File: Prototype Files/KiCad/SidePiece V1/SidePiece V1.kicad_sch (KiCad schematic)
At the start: 32 parts, among them J1 USB_C_Receptacle_USB2.0_16P, J2 Conn_01x02, U1 RP2040, U2 NCP1117-3.3_SOT223, U3 W25Q128JVS, Y1 ABM8-272-T3

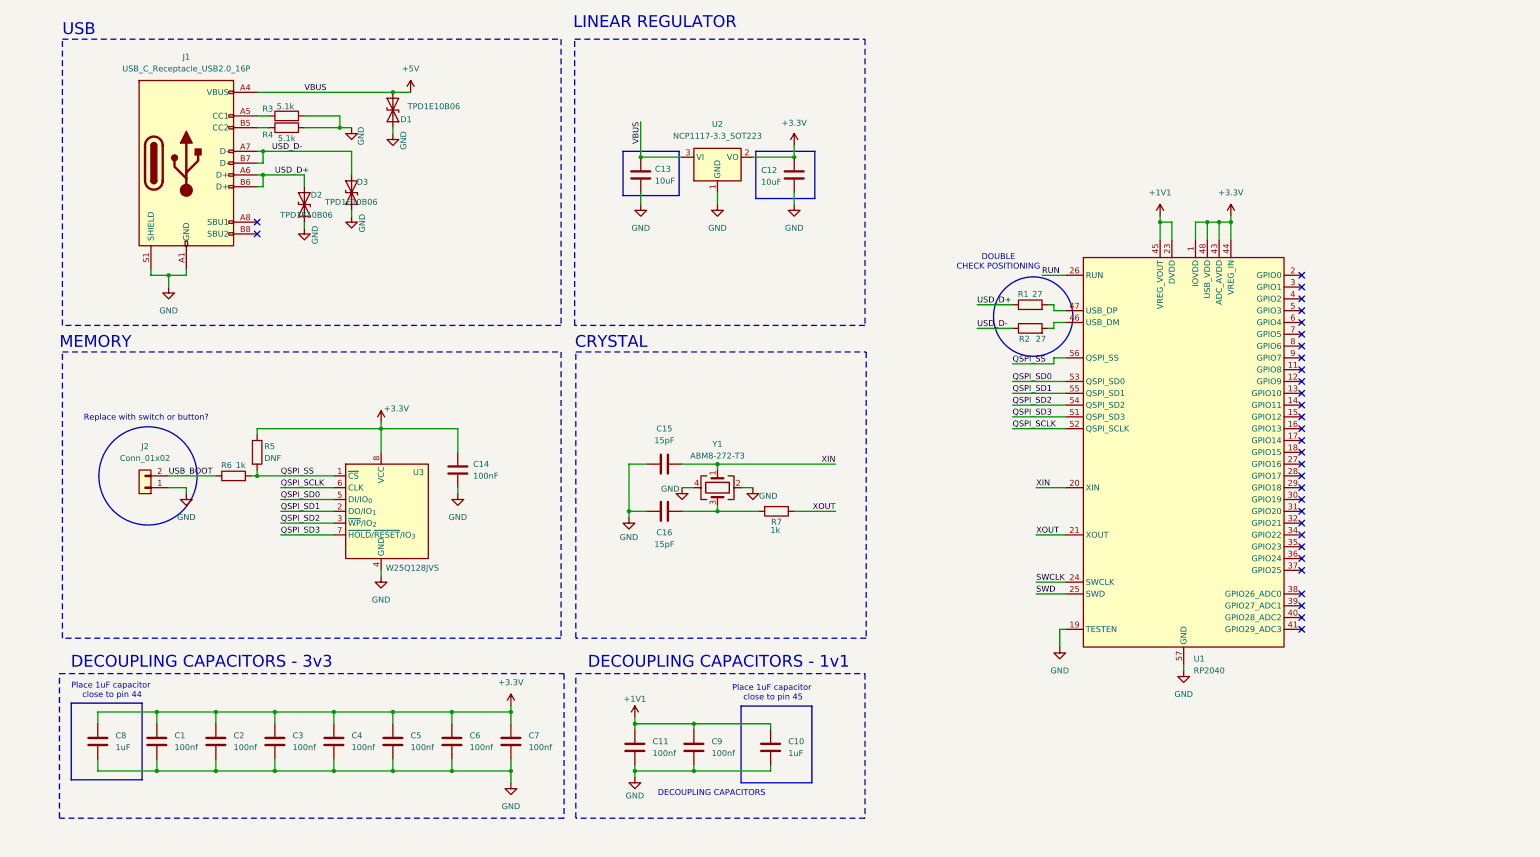
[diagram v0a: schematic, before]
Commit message: PCB Stuff
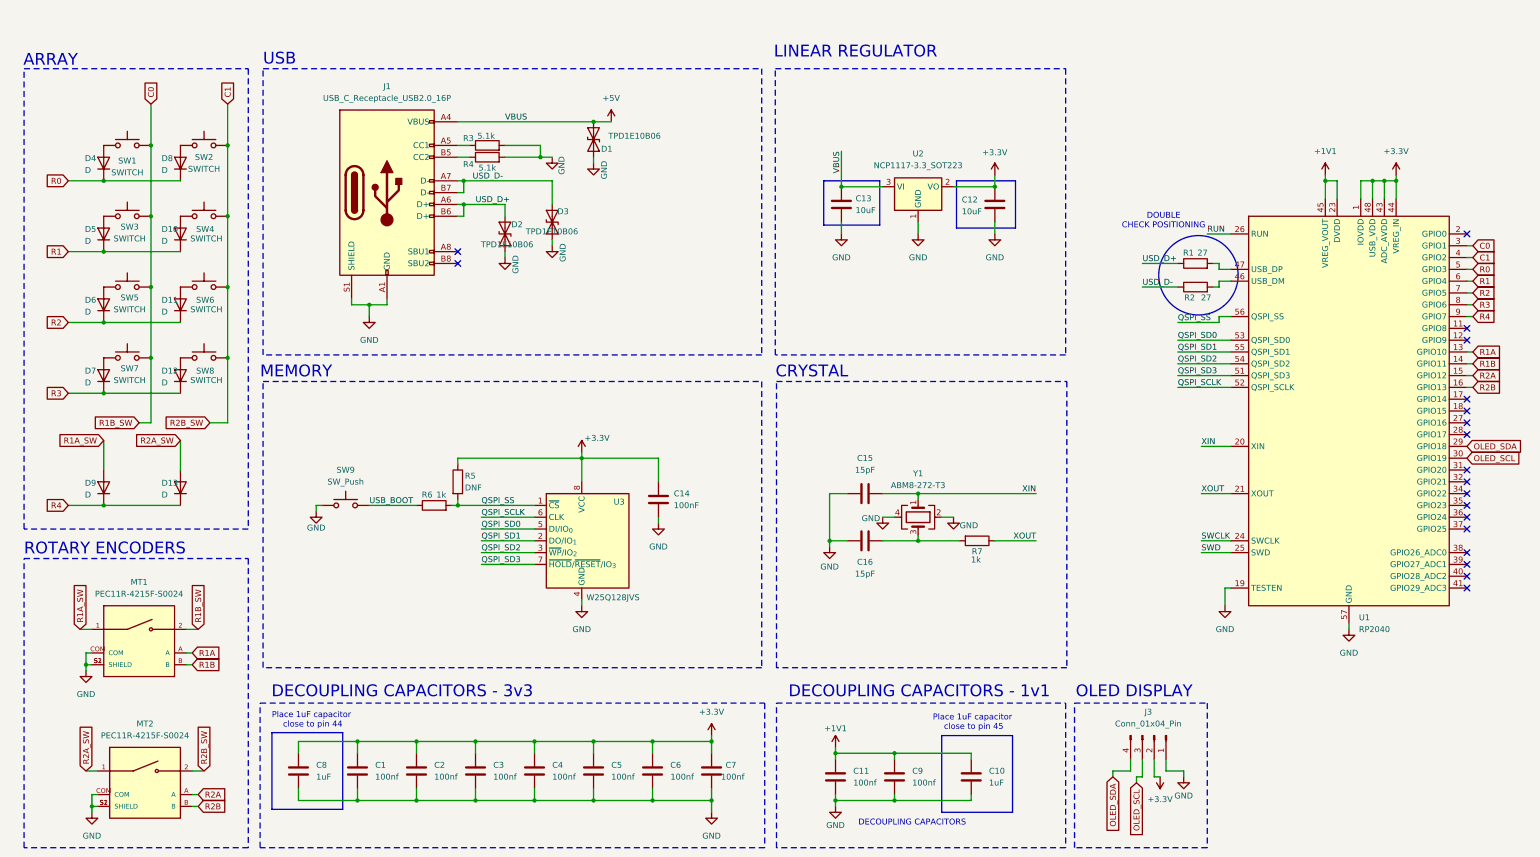
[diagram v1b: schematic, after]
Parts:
- removed J2: Conn_01x02, symbol Connector_Generic:Conn_01x02
- added D10, D11, D12, D13, D4, D5, D6, D7, D8, D9: D, Diode_SMD:D_0603_1608Metric, symbol Device:D
- added J3: Conn_01x04_Pin, 1_my_custom_libary_pretty:OLED, symbol Connector:Conn_01x04_Pin
- added MT1, MT2: PEC11R-4215F-S0024, 1_my_custom_libary_pretty:XDCR_PEC11R-4215F-S0024, symbol 1_my_custom_symbol_library:PEC11R-4215F-S0024
- added SW1, SW2, SW3, SW4, SW5, SW6, SW7, SW8: SWITCH, 1_my_custom_libary_pretty:Kailh_socket_PG1350, symbol Switch:SW_Omron_B3FS
- added SW9: SW_Push, 1_my_custom_libary_pretty:SW_SPST_PTS810, symbol Switch:SW_Push
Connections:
- net +3.3V: now also J3.2 (Pin_2)
- net GND: now also J3.1 (Pin_1), MT1.COM, MT1.S1 (SHIELD), MT1.S2 (SHIELD), MT2.COM, MT2.S1 (SHIELD), MT2.S2 (SHIELD), SW9.1
- net USB_BOOT: now also SW9.2
- net R1A: now reaches U1.13 (GPIO10)
- net R1A: now also MT1.A
- net R1B: now reaches U1.14 (GPIO11)
- net R1B: now also MT1.B
- net R2A: now reaches U1.15 (GPIO12)
- net R2A: now also MT2.A
- net R2B: now reaches U1.16 (GPIO13)
- net R2B: now also MT2.B
- net OLED_SDA: now reaches U1.29 (GPIO18)
- net OLED_SDA: now also J3.4 (Pin_4)
- net C0: now reaches U1.3 (GPIO1)
- net C0: now also MT1.2, SW1.2, SW3.2, SW5.2, SW7.2
- net OLED_SCL: now reaches U1.30 (GPIO19)
- net OLED_SCL: now also J3.3 (Pin_3)
- net C1: now reaches U1.4 (GPIO2)
- net C1: now also MT2.2, SW2.2, SW4.2, SW6.2, SW8.2
- net R0: now reaches U1.5 (GPIO3)
- net R0: now also D4.1 (K), D8.1 (K)
- net R1: now reaches U1.6 (GPIO4)
- net R1: now also D10.1 (K), D5.1 (K)
- net R2: now reaches U1.7 (GPIO5)
- net R2: now also D11.1 (K), D6.1 (K)
- net R3: now reaches U1.8 (GPIO6)
- net R3: now also D12.1 (K), D7.1 (K)
- net R4: now reaches U1.9 (GPIO7)
- net R4: now also D13.1 (K), D9.1 (K)
- new net: D4.2 (A), SW1.1
- new net: D11.2 (A), SW6.1
- new net: D12.2 (A), SW8.1
- new net: D8.2 (A), SW2.1
- new net: D10.2 (A), SW4.1
- new net: D7.2 (A), SW7.1
- new net: D6.2 (A), SW5.1
- new net: D5.2 (A), SW3.1
- new net R1A_SW: D9.2 (A), MT1.1
- new net R2A_SW: D13.2 (A), MT2.1
- no-connect marks 32 -> 19
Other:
- note added: "ARRAY"
- note added: "OLED DISPLAY"
- note added: "ROTARY ENCODERS"
- note removed: "Replace with switch or button?"
- moved on the sheet: C1, C10, C11, C12, C13, C14, C15, C16, C2, C3, C4, C5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
